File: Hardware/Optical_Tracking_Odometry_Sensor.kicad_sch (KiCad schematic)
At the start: 35 parts, among them J3 CONN_06NO_SILK_NO_POP, Q1 100mA/20V/3.8Ω, Q2 100mA/20V/3.8Ω, U1 PAA5160E1-Q, U2 LSM6DS0, U3 STM32C011F6U6, U4 RT9080-18GJ5

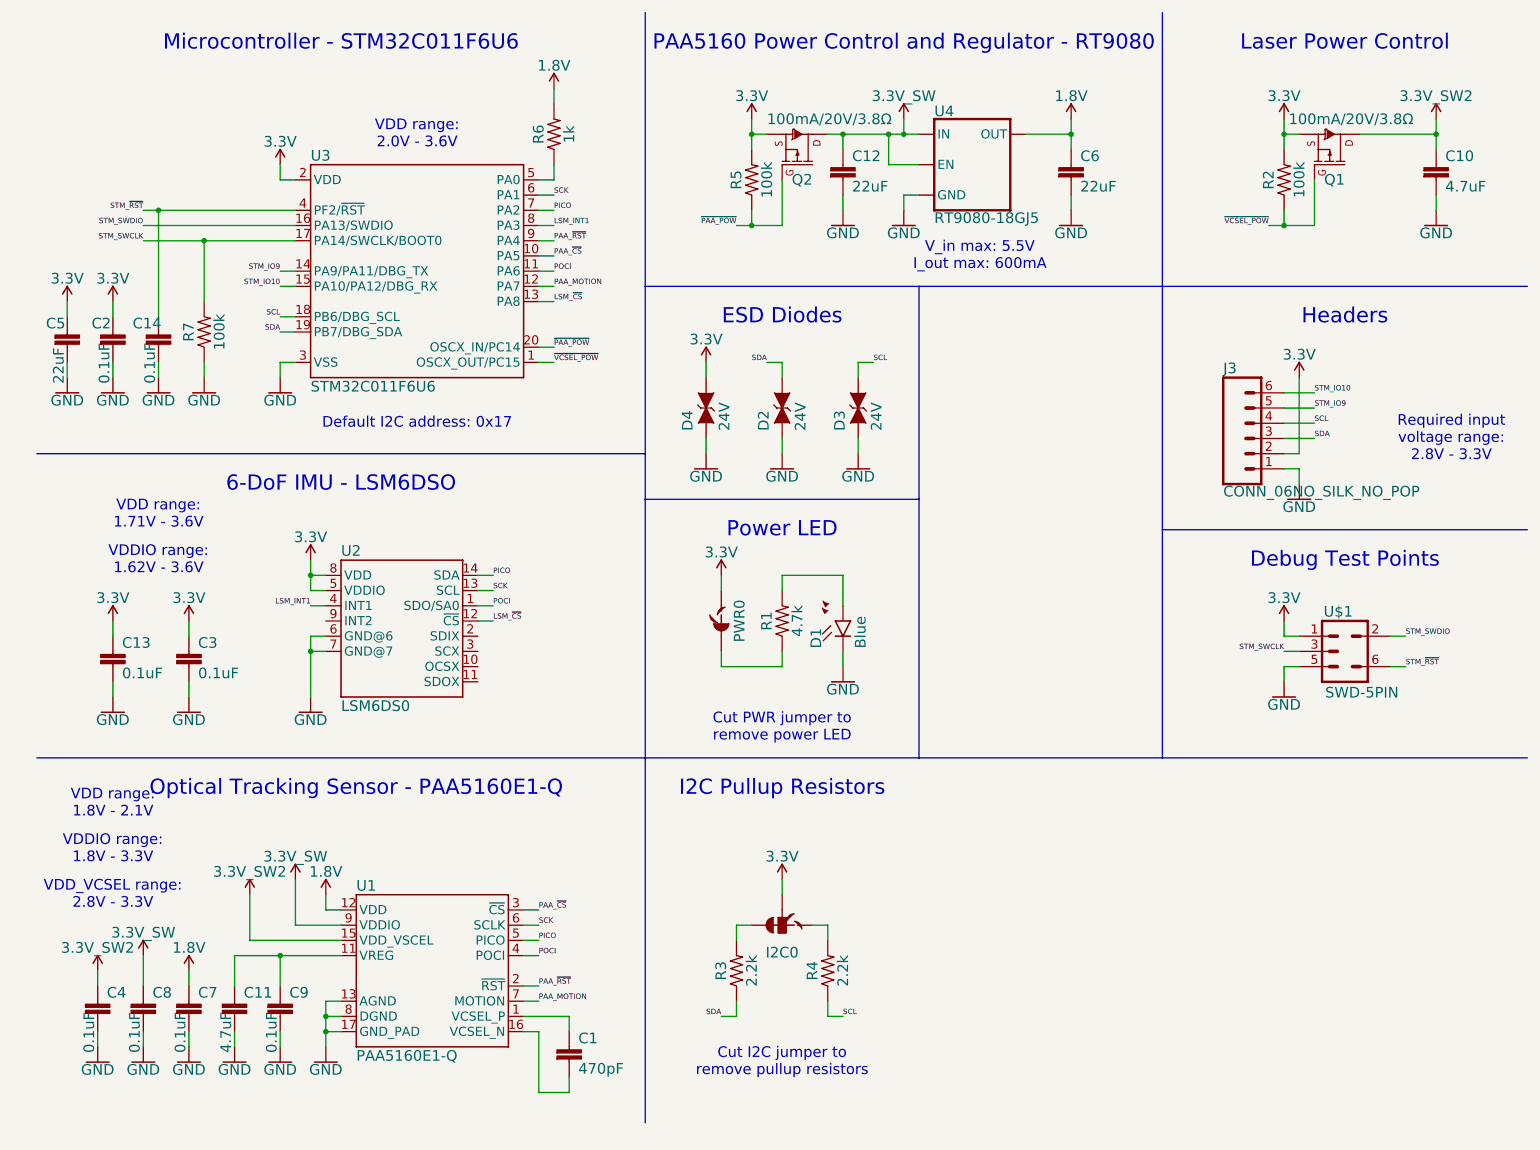
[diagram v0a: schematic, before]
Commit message: yepyep
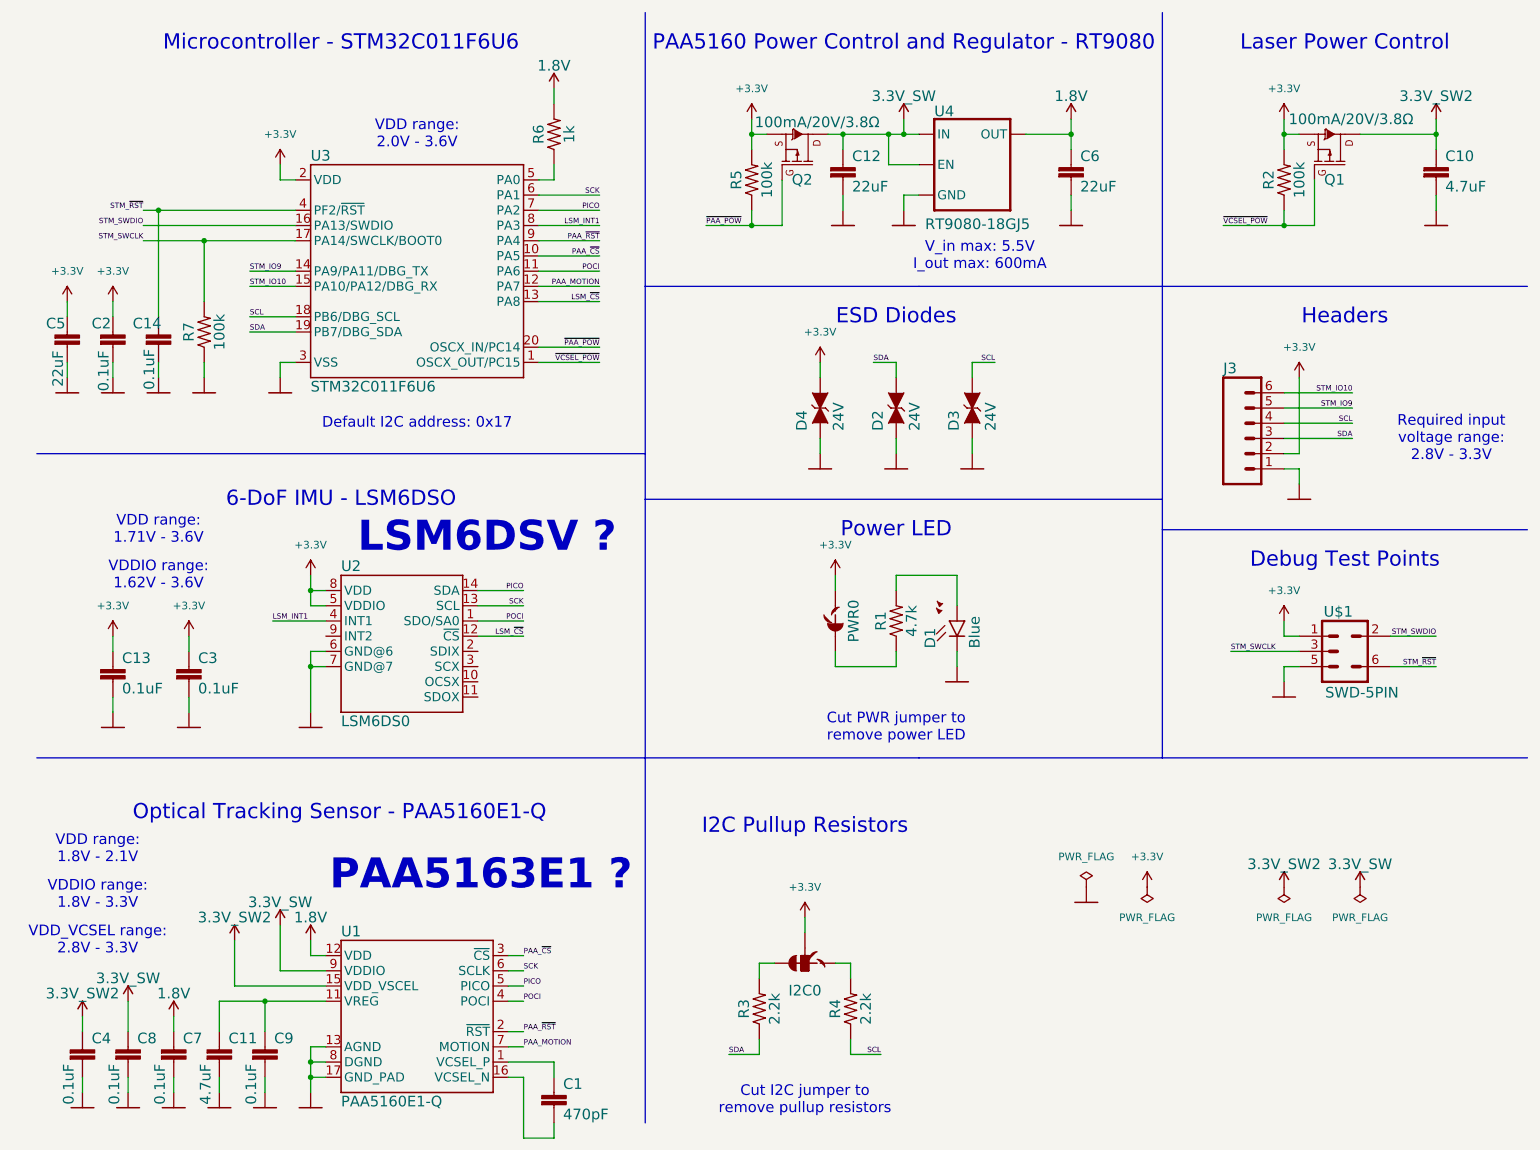
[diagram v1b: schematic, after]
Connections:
- net 3.3V renamed +3.3V
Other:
- note added: "LSM6DSV ?"
- note added: "PAA5163E1 ?"
- moved on the sheet: C1, C11, C13, C3, C4, C7, C8, C9, D1, D2, D3, D4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
